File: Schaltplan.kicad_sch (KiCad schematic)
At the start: 17 parts, among them K1 Relay, P1 USB Port vorheriger, P2 USB Port nächster, P4 USB Port Laden, U1 DC DC Wandler, U2 DC DC Wandler, U3 DS18B20, U4 Display, U5 DC DC Wandler, U6 Digitaler Poti, U7 Digitaler Poti, U8 Amperemeter, U9 DS18B20

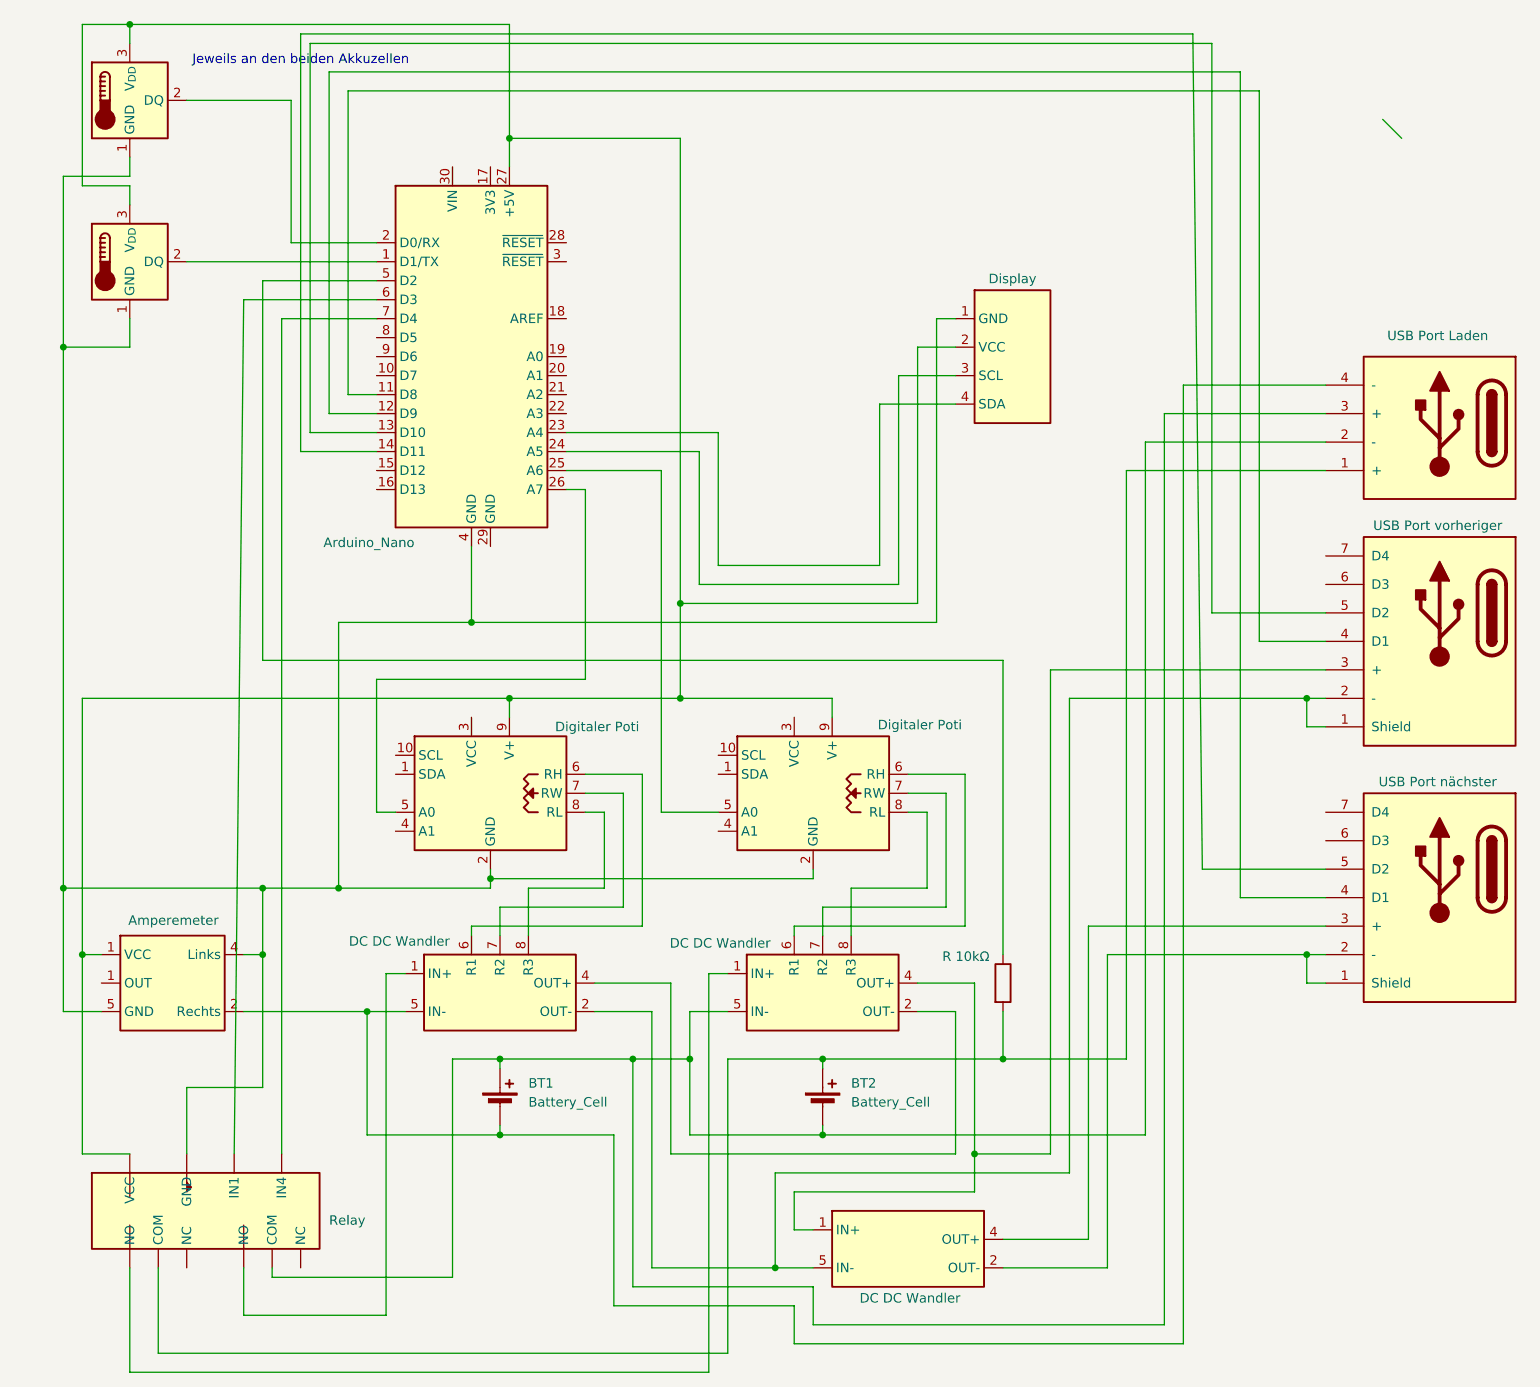
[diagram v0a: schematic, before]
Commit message: Cable moved
Co-authored-by: JumpStone <hi@jumpstone4477.de>
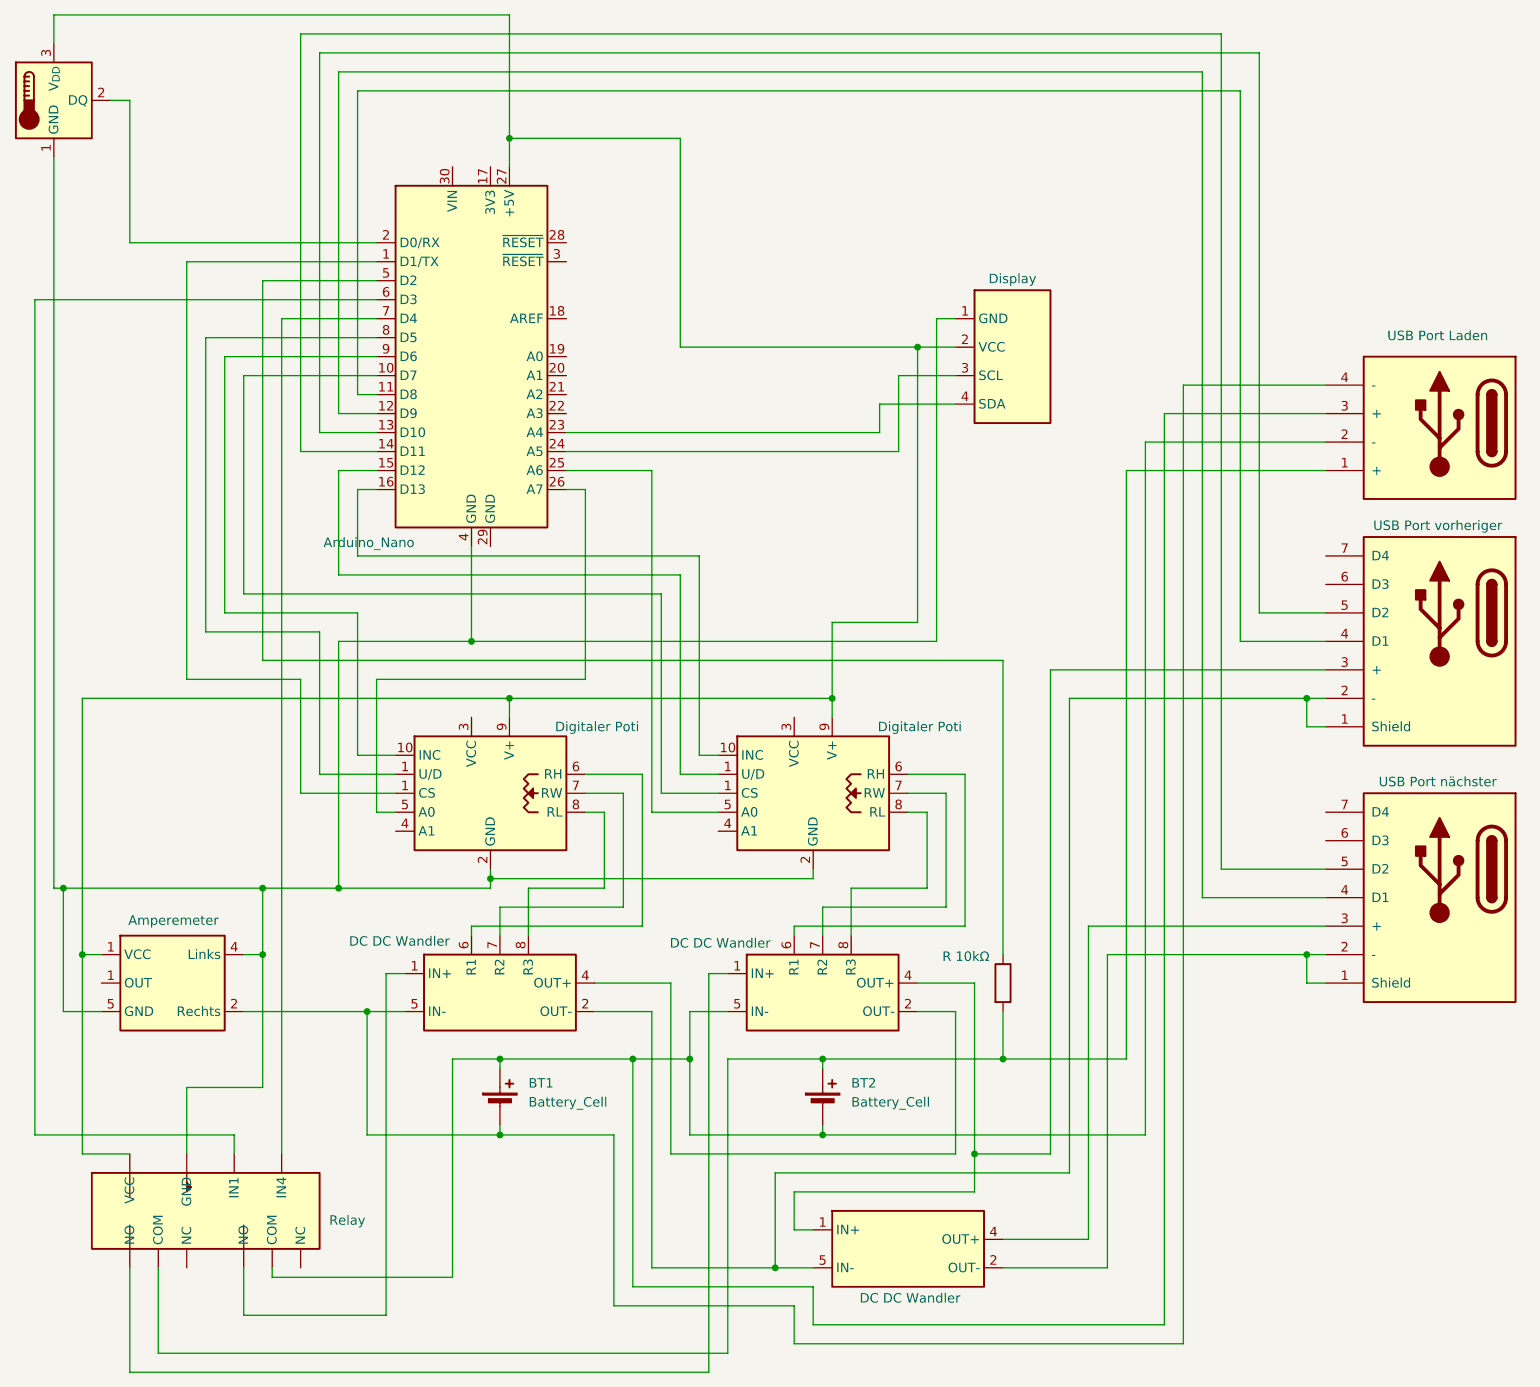
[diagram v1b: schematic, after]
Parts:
- removed U3: DS18B20, Package_TO_SOT_THT:TO-92_Inline, symbol Sensor_Temperature:DS18B20
- removed U6: Digitaler Poti, Package_SO:MSOP-10_3x3mm_P0.5mm, symbol Potentiometer_Digital:DS3502
- added U3: Digitaler Poti, Package_SO:MSOP-10_3x3mm_P0.5mm, symbol Potentiometer_Digital:DS3502
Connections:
- net at A1.4 (GND), K1. (NC), U4.1 (GND)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: now also U3.2 (GND)
- net at A1.1 (D1/TX): now also U7.1 (CS)
- net at A1.27 (+5V), K1. (NC), U4.2 (VCC)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: now also U3.9 (V+)
- net at U7.1 (CS): now also A1.8 (D5)
- net at U7.10 (INC): now also A1.9 (D6)
- net at K1. (NC): now also A1.7 (D4)
- net at A1.25 (A6): now also U3.5 (A0)
- net at U1.6 (R1): now also U3.6 (RH)
- net at U1.7 (R2): now also U3.7 (RW)
- net at U1.8 (R3): now also U3.8 (RL)
- net at A1.10 (D7): now also U3.1 (CS)
- net at A1.15 (D12): now also U3.1 (CS)
- net at A1.16 (D13): now also U3.10 (INC)
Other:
- note removed: "Jeweils an den beiden Akkuzellen"
